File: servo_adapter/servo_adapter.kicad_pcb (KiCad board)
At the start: 4 copper layers, 64 x 50 mm, 17 parts, among them J1 T4140012081-000, J2 Conn_01x10_Socket, J4 T4141012051-000, U1 MUN5233T1G, U2 MUN5233T1G, U3 MUN5233T1G, U4 MUN5233T1G

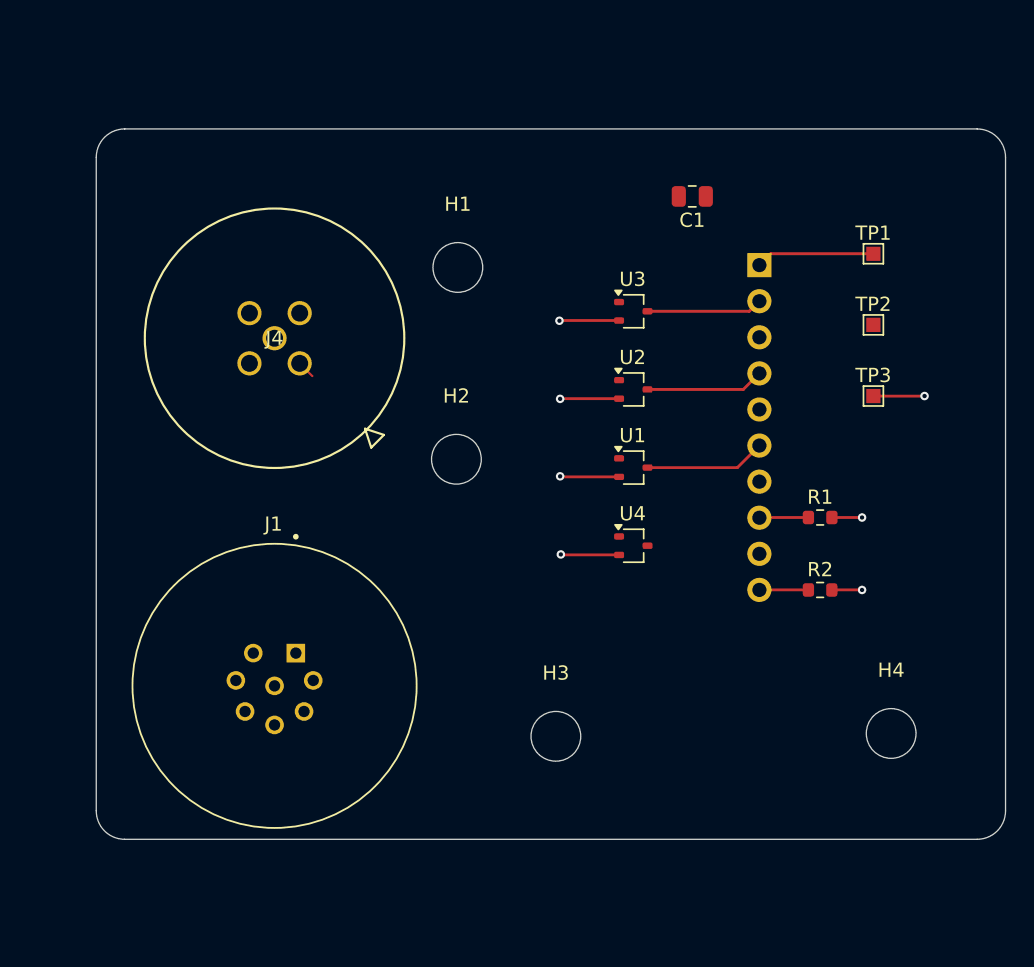
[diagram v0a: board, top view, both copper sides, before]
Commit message: Refactored the dimensions and footprints
+ Re-dimensioned the step file.
+ Relocated the 2.54mm du-pont connector/socket.
+ Changed the MH3 and MH4 to use 2.2mm holes.(closest to 2.0mm).
+ Relocated MH1 and MH2
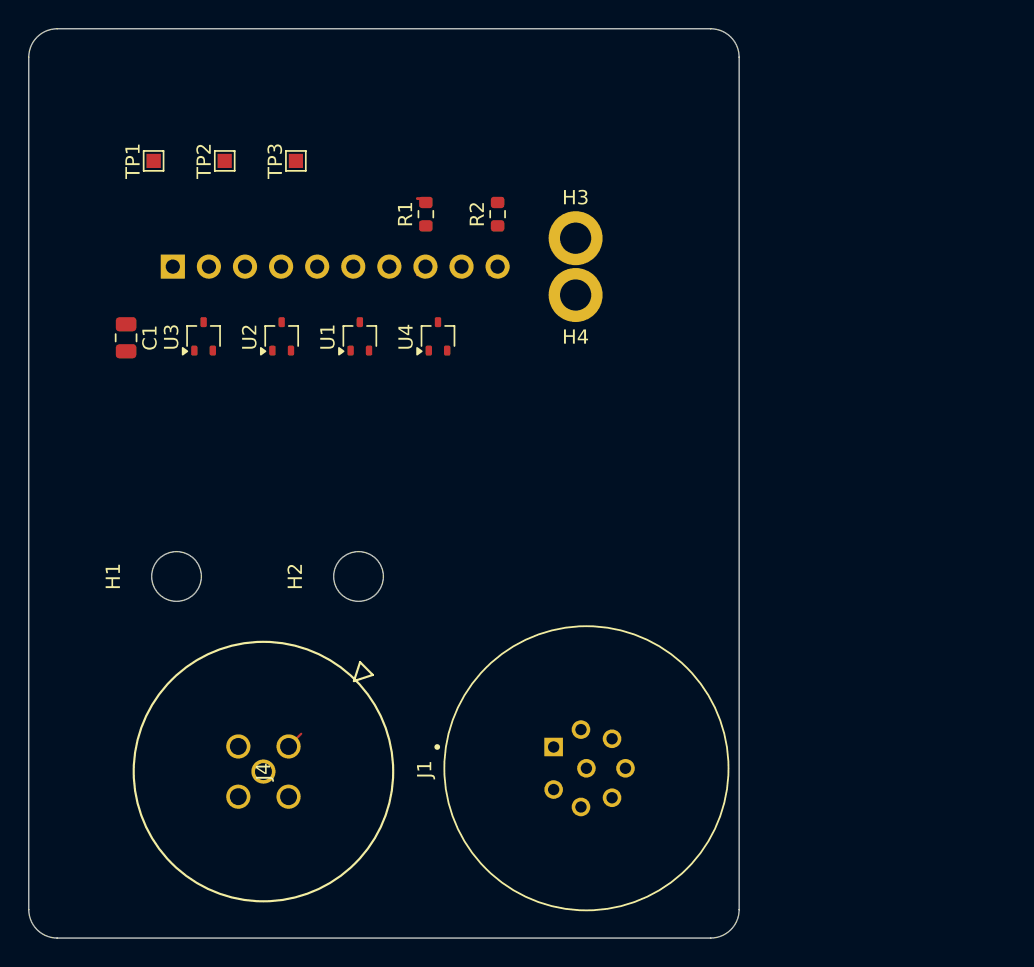
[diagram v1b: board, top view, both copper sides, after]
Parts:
- H3, H4: footprint MountingHole:MountingHole_3.5mm -> MountingHole:MountingHole_2.2mm_M2_DIN965_Pad
- moved TP1 51.1 mm to (104.0, 52.2), turned to 90 degrees
- moved TP2 47.1 mm to (109.0, 52.2), turned to 90 degrees
- moved TP3 43.9 mm to (114.0, 52.2), turned to 90 degrees
- moved J2 41.3 mm to (105.4, 59.7), turned to -90 degrees
- moved C1 41.1 mm to (102.1, 64.7), turned to -90 degrees
- moved H4 38.0 mm to (133.7, 61.7)
- moved H3 35.1 mm to (133.7, 57.7)
- moved R1 35.0 mm to (123.2, 56.0), turned to 90 degrees
- moved R2 34.9 mm to (128.2, 56.0), turned to 90 degrees
- moved J4 34.0 mm to (110.0, 97.0), turned to 90 degrees
- moved U3 30.3 mm to (107.6, 64.6), turned to 90 degrees
- moved H1 29.4 mm to (105.7, 81.5), turned to 90 degrees
- moved U2 25.0 mm to (113.1, 64.6), turned to 90 degrees
- moved J1 22.7 mm to (134.5, 95.0), turned to 90 degrees
- moved U1 21.3 mm to (118.6, 64.6), turned to 90 degrees
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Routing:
- net GND: track 24.8 -> 0.71 mm, vias 7 -> 0
- net /ENA-: track 8.52 -> 0.00 mm
- net /+5V_Servo: track 8.36 -> 0.00 mm
- net /DIR-: track 8.34 -> 0.00 mm
- net /PUL-: track 8.17 -> 0.00 mm
- net /ALARM_OUT: track 3.45 -> 0.01 mm
- net /PED-: track 3.46 -> 0.02 mm
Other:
- board size 64 x 50 mm -> 50 x 64 mm
